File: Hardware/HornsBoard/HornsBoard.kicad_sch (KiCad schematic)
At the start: 4 parts, among them J1 Conn_01x03, J2 Conn_01x02, J3 Conn_01x02, J4 Conn_01x02

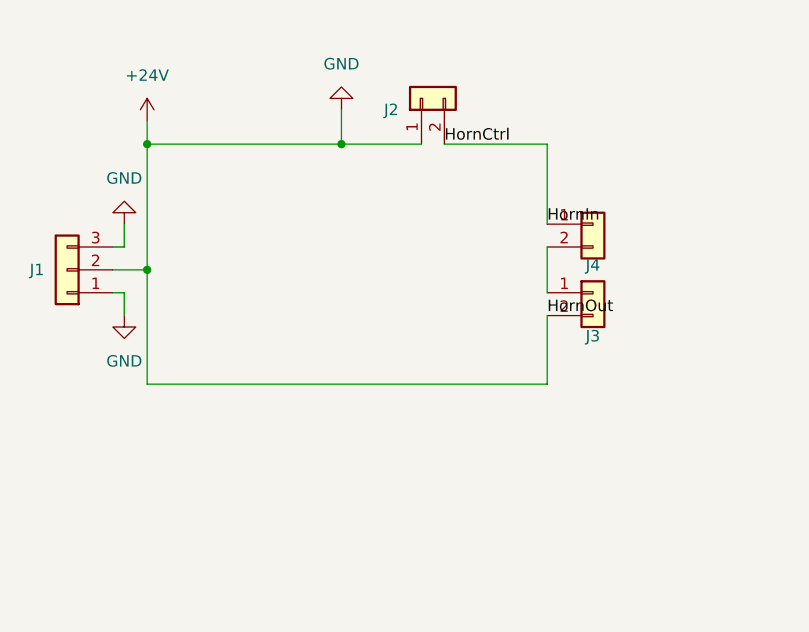
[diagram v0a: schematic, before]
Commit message: Finished Horns Board Project
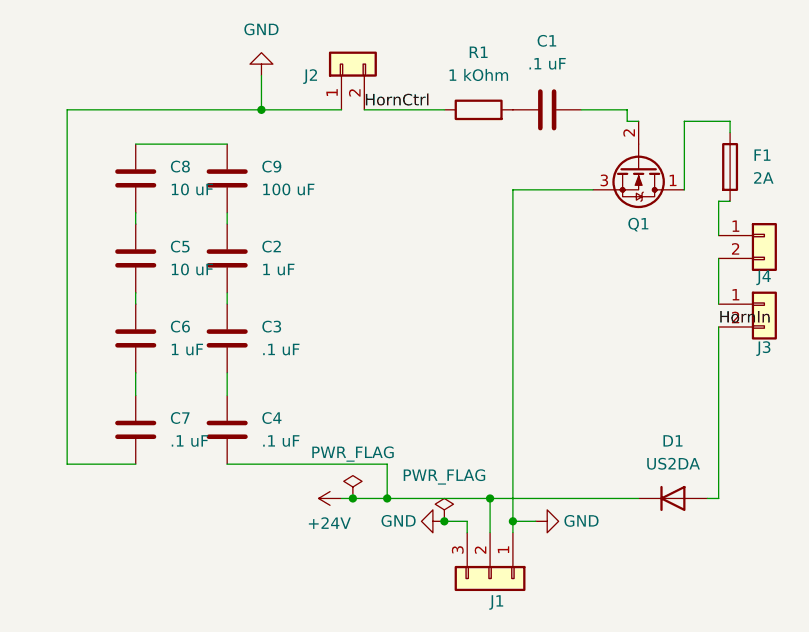
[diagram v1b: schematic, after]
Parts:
- added C1, C3, C4, C7: .1 uF, Capacitor_SMD:CP_Elec_4x4.5, symbol device:C
- added C2, C6: 1 uF, Capacitor_SMD:CP_Elec_4x4.5, symbol device:C
- added C5, C8: 10 uF, Capacitor_SMD:CP_Elec_4x4.5, symbol device:C
- added C9: 100 uF, Capacitor_SMD:CP_Elec_4x4.5, symbol device:C
- added D1: US2DA, Diode_SMD:D_SMA, symbol Diode:US2DA
- added F1: 2A, Fuse:Fuse_0603_1608Metric, symbol Device:Fuse
- added Q1: BS108, Package_TO_SOT_THT:TO-92_Inline, symbol Transistor_FET:BS108
- added R1: 1 kOhm, Resistor_SMD:R_0201_0603Metric, symbol device:R
- J1: footprint (none) -> Connector_Molex:Molex_KK-396_A-41791-0003_1x03_P3.96mm_Vertical
- J2, J3, J4: footprint (none) -> Connector_Molex:Molex_KK-396_A-41791-0002_1x02_P3.96mm_Vertical
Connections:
- net +24V: now also C4.2, D1.1 (K); no longer J1.1 (Pin_1), J1.3 (Pin_3), J2.1 (Pin_1), J3.2 (Pin_2)
- net HornCtrl: now also R1.1; no longer J4.1 (Pin_1)
- new net: C2.2, C3.1
- new net: C3.2, C4.1
- new net: F1.2, J4.1 (Pin_1)
- new net: C1.1, R1.2
- new net: C1.2, Q1.2 (G)
- new net: C5.2, C6.1
- new net: C6.2, C7.1
- new net: C8.1, C9.1
- new net: C2.1, C9.2
- new net: F1.1, Q1.1 (D)
- new net: C5.1, C8.2
- new net GND: C7.2, J1.1 (Pin_1), J1.3 (Pin_3), J2.1 (Pin_1), Q1.3 (S)
- new net HornIn: D1.2 (A), J3.2 (Pin_2)
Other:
- moved on the sheet: J1, J2, J3, J4
